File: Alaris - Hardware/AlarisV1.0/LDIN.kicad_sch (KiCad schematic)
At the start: 28 parts, among them J7 USB_C_Receptacle_USB2.0_16P, SW7 SW_MEC_5G, SW8 SW_MEC_5G, U16 ESP32-C3, Y8 40MHz

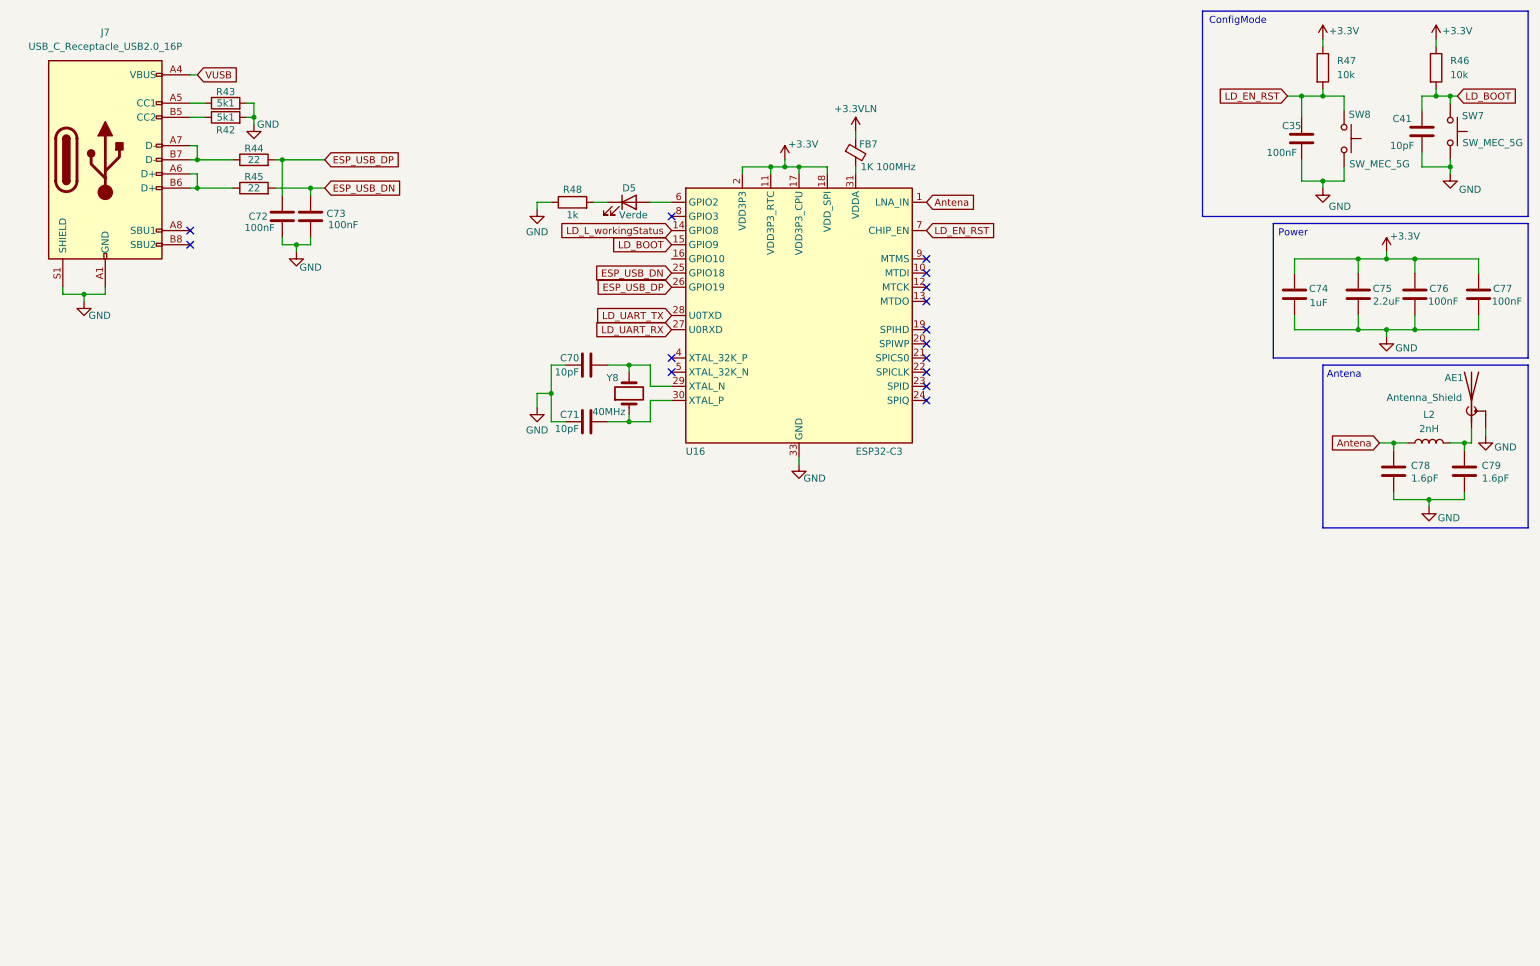
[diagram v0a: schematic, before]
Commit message: Desenvolvimento da PCB
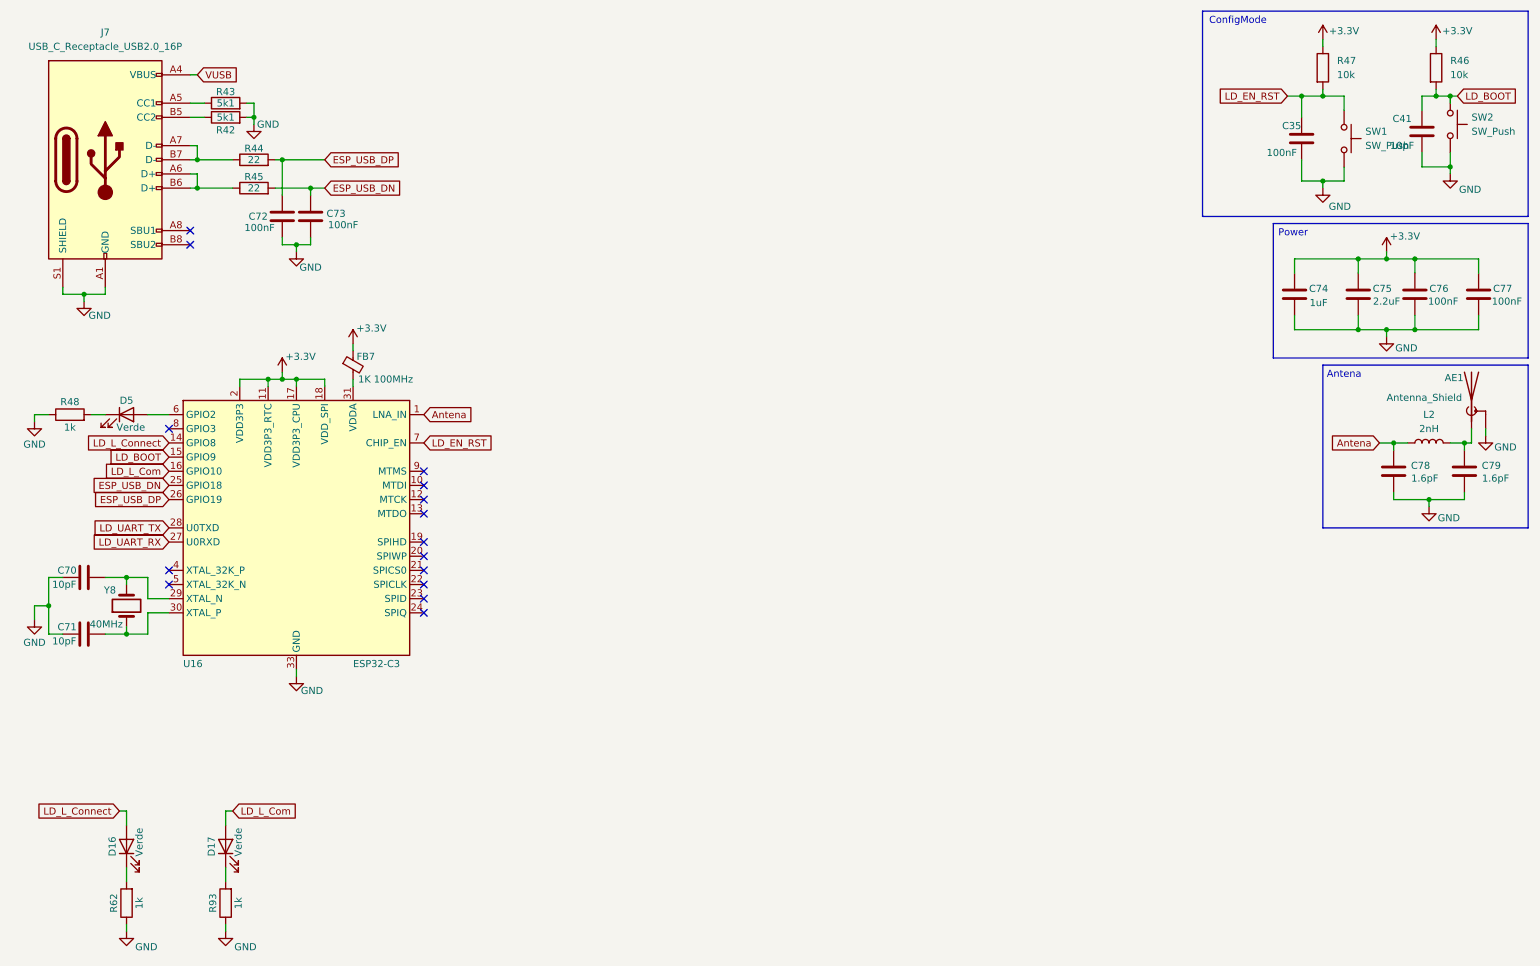
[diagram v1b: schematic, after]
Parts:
- removed SW7, SW8: SW_MEC_5G, symbol Switch:SW_MEC_5G
- added D16, D17: Verde, LED_SMD:LED_0603_1608Metric_Pad1.05x0.95mm_HandSolder, symbol Device:LED
- added R62, R93: 1k, Resistor_SMD:R_0603_1608Metric_Pad0.98x0.95mm_HandSolder, symbol Device:R
- added SW1, SW2: SW_Push, Footprint:SKRK, symbol Cleber:SW_Push
- D5: footprint (none) -> LED_SMD:LED_0603_1608Metric_Pad1.05x0.95mm_HandSolder
- FB7: footprint (none) -> Capacitor_SMD:C_0603_1608Metric_Pad1.08x0.95mm_HandSolder
- L2: footprint (none) -> Inductor_SMD:L_0603_1608Metric_Pad1.05x0.95mm_HandSolder
- R42, R43, R44, R45, R48: footprint (none) -> Resistor_SMD:R_0603_1608Metric_Pad0.98x0.95mm_HandSolder
- Y8: footprint Crystal:Crystal_SMD_0603-4Pin_6.0x3.5mm_HandSoldering -> Crystal:Crystal_SMD_3225-4Pin_3.2x2.5mm
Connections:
- net +3.3VLN is gone; now on net +3.3V: FB7.1
- net GND: now also R62.1, R93.1, SW1.2, SW2.2
- net LD_BOOT: now also SW2.1
- net LD_EN_RST: now also SW1.1
- net LD_L_Com: now reaches U16.16 (GPIO10)
- net LD_L_Com: now also D17.2 (A)
- net LD_L_workingStatus renamed LD_L_Connect
- net LD_L_Connect: now also D16.2 (A)
- new net: D16.1 (K), R62.2
- new net: D17.1 (K), R93.2
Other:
- moved on the sheet: C70, C71, D5, FB7, R48, U16, Y8
